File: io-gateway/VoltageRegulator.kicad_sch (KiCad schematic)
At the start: 16 parts, among them U3 TPS54308

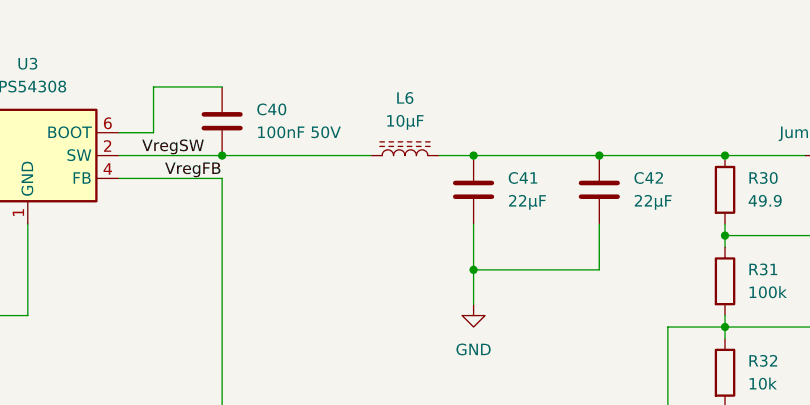
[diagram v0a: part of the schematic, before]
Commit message: V1.2
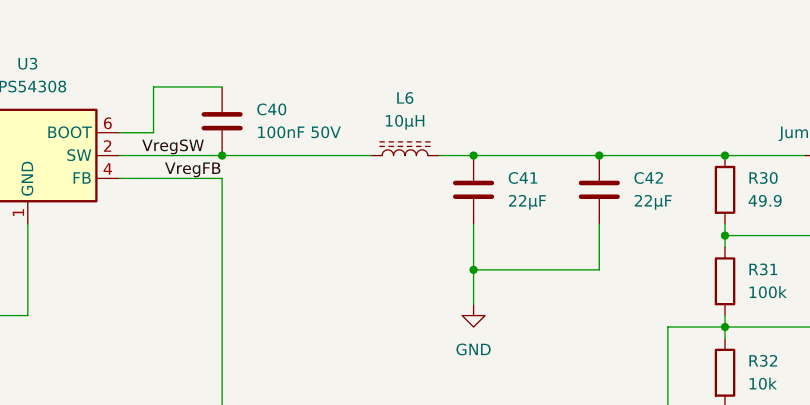
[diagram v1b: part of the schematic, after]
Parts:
- L6: value 10µF -> 10µH
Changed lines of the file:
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@@
 			)
 		)
-		(property "Value" "10µF"
+		(property "Value" "10µH"
 			(at 139.7 57.15 90)
 			(effects
